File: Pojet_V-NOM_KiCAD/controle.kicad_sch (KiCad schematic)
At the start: 12 parts, among them U1 STM32G431CBU6, Y1 16 MHz

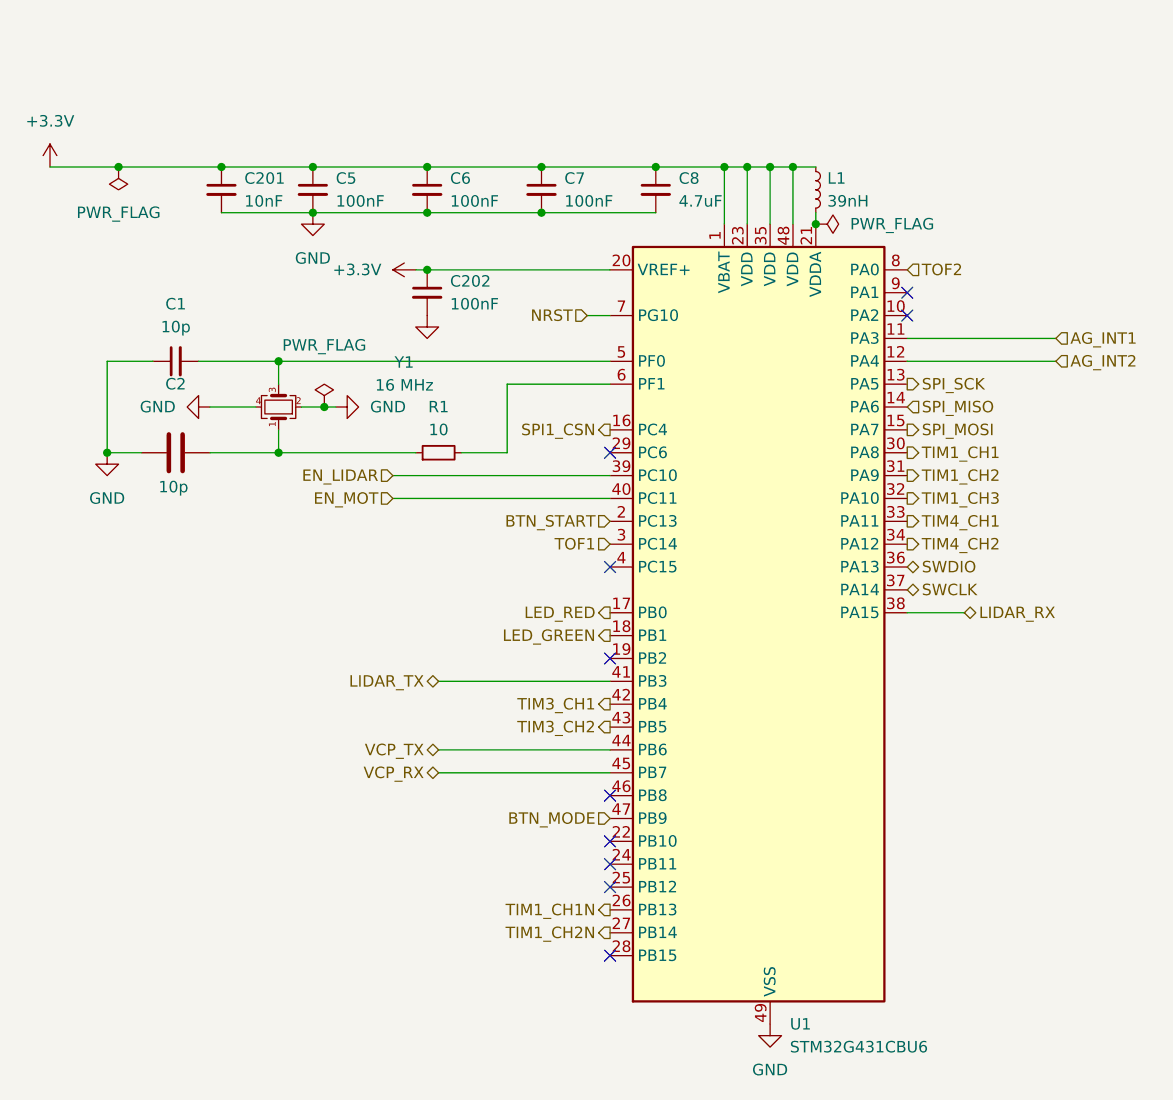
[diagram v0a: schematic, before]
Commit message: maj final aprés correction du prof + logo ensea
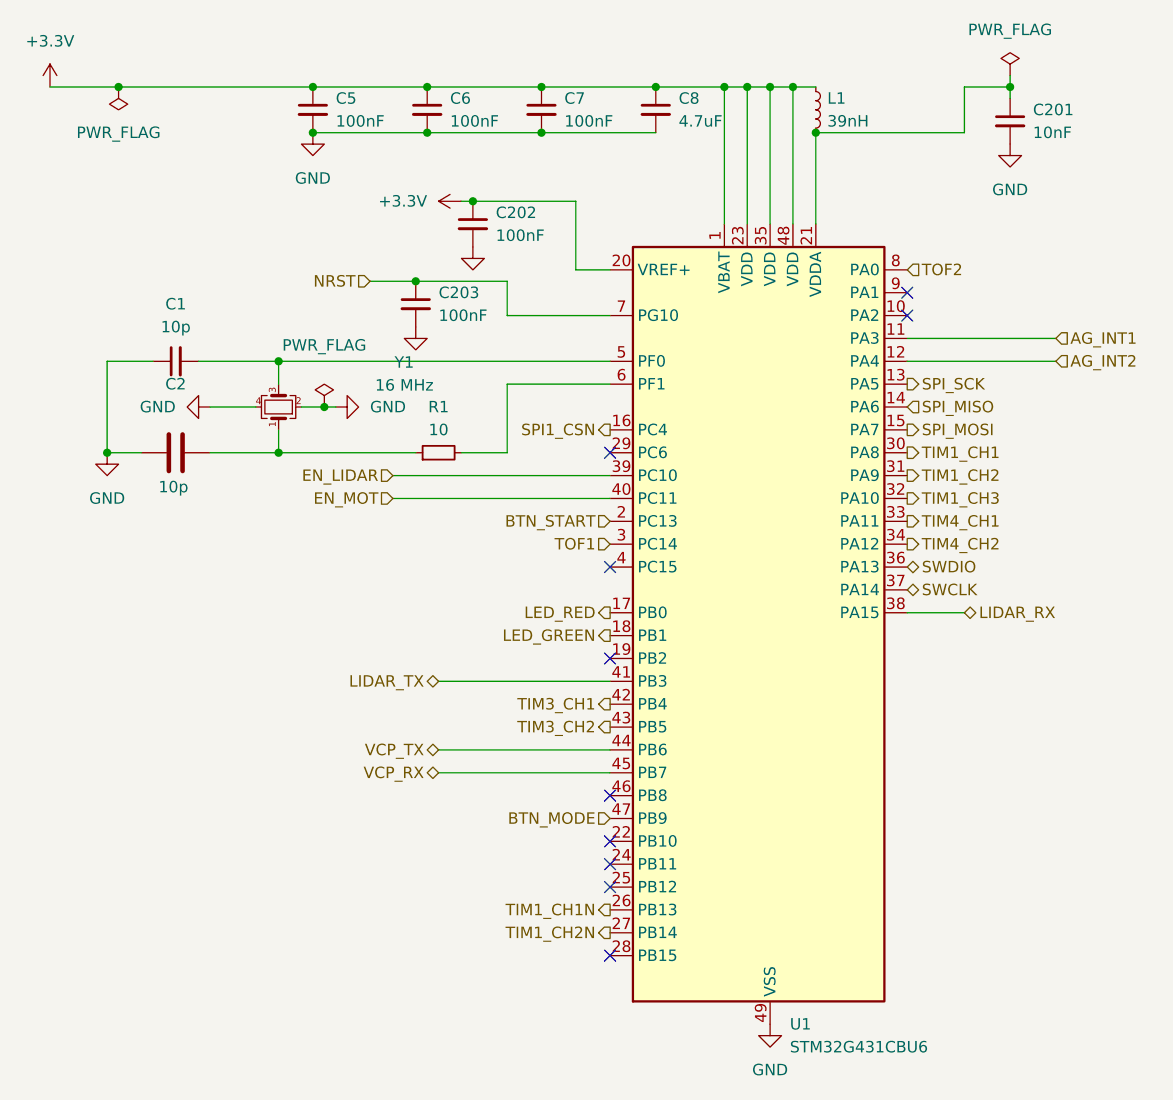
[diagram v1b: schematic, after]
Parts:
- added C203: 100nF, Capacitor_SMD:C_0402_1005Metric, symbol Device:C_Small
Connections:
- net +3.3V: no longer C201.1
- net GND: now also C203.2
- net NRST: now also C203.1
- net at L1.2, U1.21 (VDDA): now also C201.1
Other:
- moved on the sheet: C201, C202, C5, C6, C7, C8, L1
